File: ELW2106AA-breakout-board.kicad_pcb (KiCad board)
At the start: 2 copper layers, 77 x 18 mm, 28 parts, among them J1 Conn_02x04_Male-custom, U1 TLV61046ADB, U2 XC6206P332MR, U3 TXS0108EPW

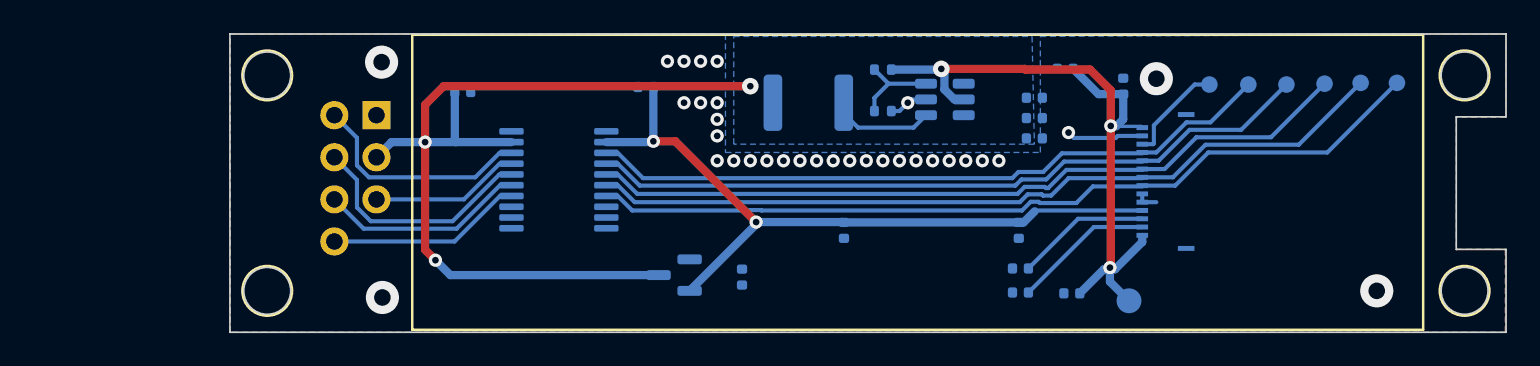
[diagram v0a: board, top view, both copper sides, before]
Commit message: third revision
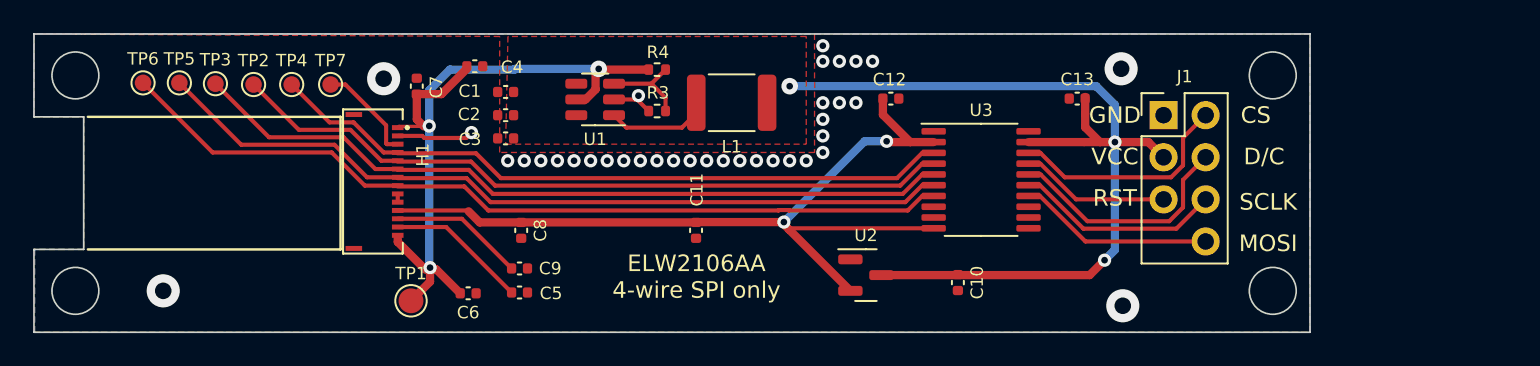
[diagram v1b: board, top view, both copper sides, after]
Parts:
- C1, C10, C11, C12, C13, C2, C3, C4, C5, C6, C7, C8, C9, H1, J1, L1, R3, R4, TP1, TP2, TP3, TP4, TP5, TP6, TP7, U1, U2, U3: moved to F.Cu
- moved TP6 75.7 mm to (81.8, 102.0), turned to 0 degrees
- moved TP5 71.3 mm to (83.9, 102.0), turned to 0 degrees
- moved TP3 66.9 mm to (86.1, 102.0), turned to 0 degrees
- moved TP2 62.3 mm to (88.4, 102.0), turned to 0 degrees
- moved TP4 57.7 mm to (90.7, 102.0), turned to 0 degrees
- moved TP7 53.0 mm to (93.1, 102.0), turned to 0 degrees
- moved H1 47.9 mm to (95.6, 107.9)
- moved J1 47.5 mm to (143.3, 103.9), turned to 0 degrees
- moved TP1 43.3 mm to (97.9, 115.1), turned to 0 degrees
- moved C7 42.6 mm to (98.3, 102.2)
- moved C13 37.1 mm to (138.1, 102.9), turned to 0 degrees
- moved C6 36.4 mm to (101.4, 114.7), turned to 180 degrees
- moved C4 35.6 mm to (101.8, 101.0), turned to 180 degrees
- moved C1 31.9 mm to (103.6, 102.5), turned to 0 degrees
- moved C2 31.9 mm to (103.6, 103.9), turned to 0 degrees
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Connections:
- U3 pad 10: unconnected-(U3-Pad10) -> +3V3
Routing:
- net +3V3: track 43.7 -> 52.5 mm
- net GND: track 8.37 -> 7.89 mm, vias 33 -> 36
- added copper zone on F.Cu, net VCC
- removed copper zone on B.Cu, net VCC
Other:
- outline, holes or cut-outs redrawn
- board text added: "CS"
- board text added: "D/C"
- board text added: "ELW2106AA 4-wire SPI only"
- board text added: "GND"
- board text added: "MOSI"
- board text added: "RST"
- board text added: "SCLK"
- board text added: "VCC"
